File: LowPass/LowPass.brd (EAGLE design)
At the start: 50.8 x 17.4 mm, 10 parts

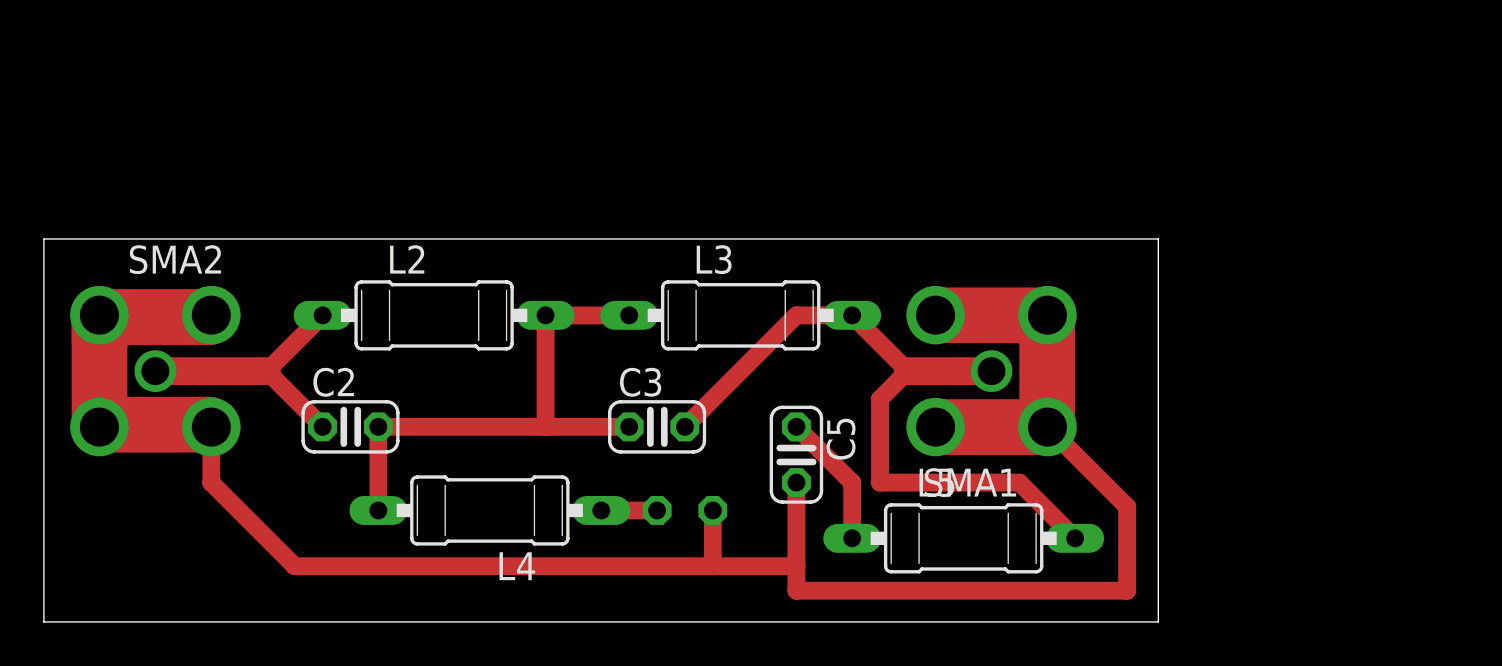
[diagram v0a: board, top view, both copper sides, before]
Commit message: Version SMD Reject Band
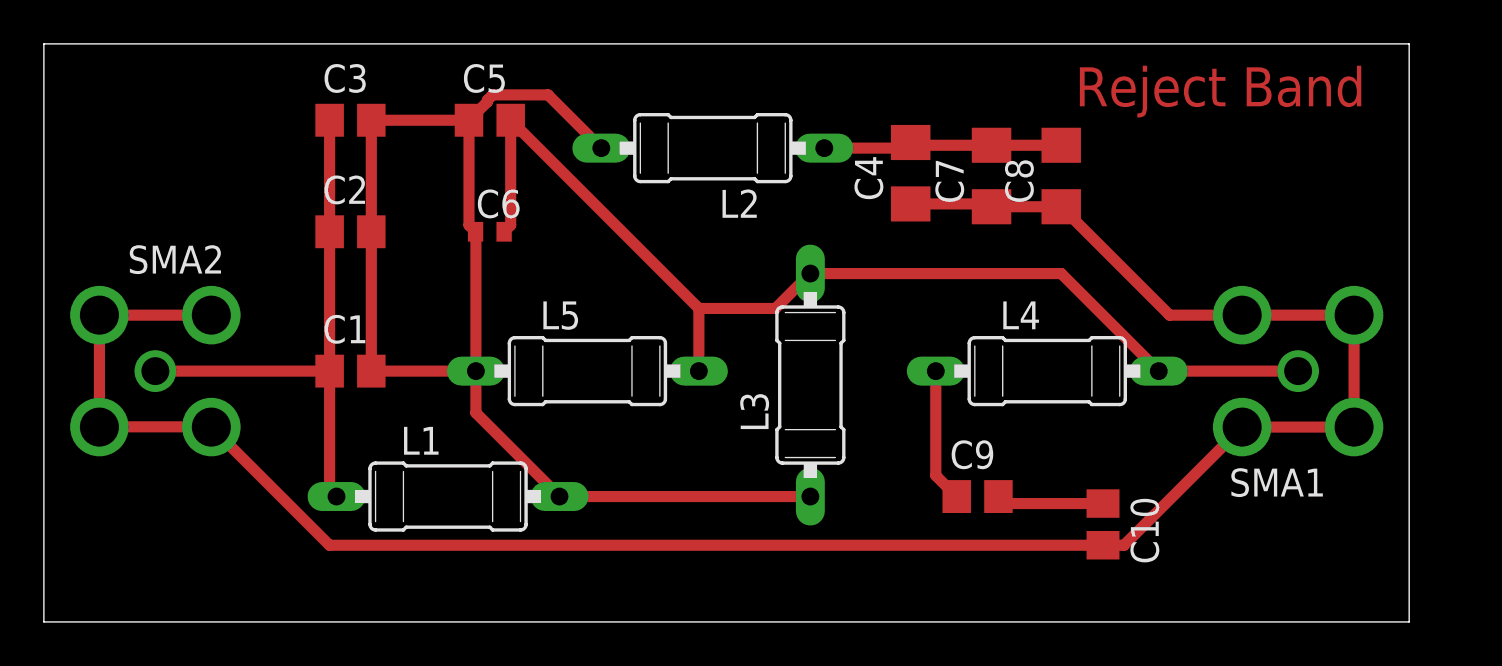
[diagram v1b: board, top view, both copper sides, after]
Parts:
- added C1: 100p, rcl:C0805
- added C10, C9: 10p, rcl:C0805
- added C6: 68p, rcl:C0402
- added C7, C8: 4p, rcl:C1206
- added L1: 12n, inductors:MICC10
- C2: value (none) -> 100p; device rcl:C025-024X044 -> rcl:C0805
- C3: value (none) -> 10p; device rcl:C025-024X044 -> rcl:C0805
- C4: value (none) -> 4p; device rcl:C025-024X044 -> rcl:C1206
- C5: value (none) -> 18p; device rcl:C025-024X044 -> rcl:C0805
- L2: value MICC10 -> 220n
- L3: value MICC10 -> 85n
- L4: value MICC10 -> 500n
- L5: value MICC10 -> 100n
- moved L4 26.2 mm to (49.5, 91.4), turned to 0 degrees
- moved C5 20.7 mm to (24.1, 102.9), turned to 0 degrees
- moved C3 19.8 mm to (17.8, 102.9)
- moved L5 18.8 mm to (28.6, 91.4)
- moved C4 18.5 mm to (43.3, 100.5), flipped to the top, turned to 90 degrees
- moved L2 14.8 mm to (34.3, 101.6), turned to 180 degrees
- moved SMA1 14.0 mm to (61.0, 91.4)
- moved C2 8.89 mm to (17.8, 97.8)
- moved L3 4.49 mm to (38.7, 90.8), turned to 90 degrees
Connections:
- removed net N$7: C3.2, L3.2, L5.2, SMA1.1
- removed net N$9: C5.1, L5.1
- new net N$10: C9.1, L4.1
- new net N$11: C10.1, C9.2
- new net N$12: C4.2, C7.2, C8.2, L2.1
- net GND: now also C10.2, C4.1, C7.1, C8.1; no longer C4.2, C5.2
- net N$3: now also C1.1, C3.1, L1.1; no longer L2.1
- net N$5: now also C1.2, C3.2, C5.1, C6.1, L1.2, L5.1; no longer C3.1, L4.2
- net N$8: now also C5.2, C6.2, L3.2, L4.2, L5.2, SMA1.1; no longer C4.1, L4.1
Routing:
- net N$8: track 2.54 -> 51.3 mm
- net N$5: track 24.2 -> 60.4 mm
- net N$7: track 32.7 -> 0.00 mm
- net N$3: track 12.3 -> 25.9 mm
- net N$12: track 0.00 -> 11.0 mm
- net GND: track 110.1 -> 99.6 mm
- net N$10: track 0.00 -> 6.75 mm
- net N$9: track 6.13 -> 0.00 mm
- net N$11: track 0.00 -> 4.90 mm
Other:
- board size 50.8 x 17.4 mm -> 62.2 x 26.3 mm
- board text added: "Reject Band"
